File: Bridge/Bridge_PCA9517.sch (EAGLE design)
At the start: 13 parts, among them IC2 SI7005, X1 SCL, X2 3v3, X3 GND, X4 SCL, X5 SDA, X6 SDA, X7 3v3, X8 GND

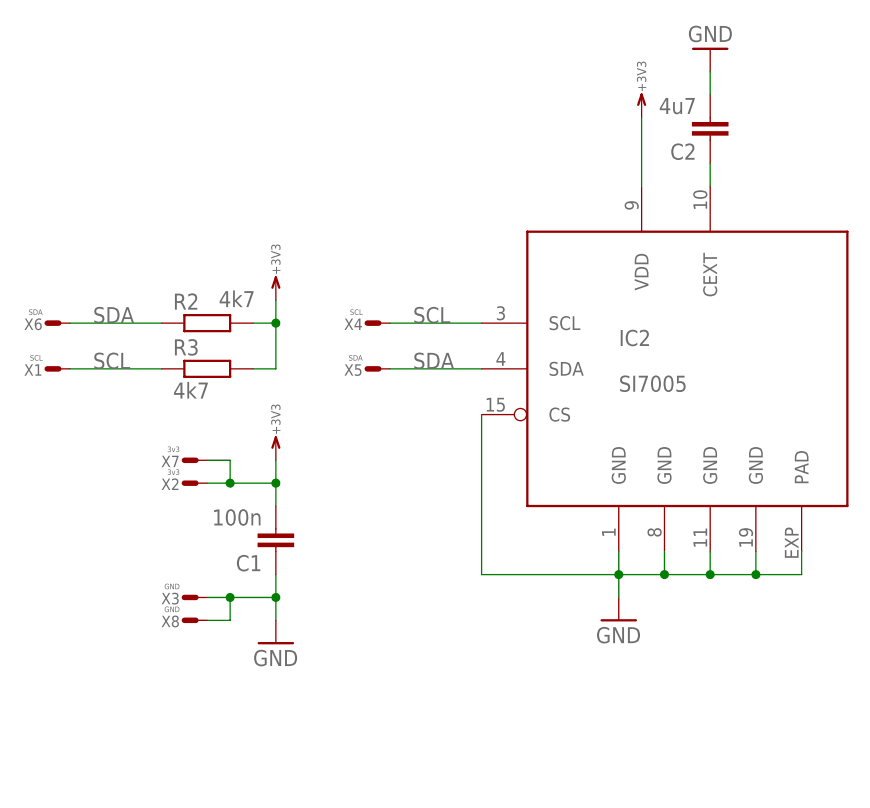
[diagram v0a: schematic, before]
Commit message: Typo correction and more elegance presentation
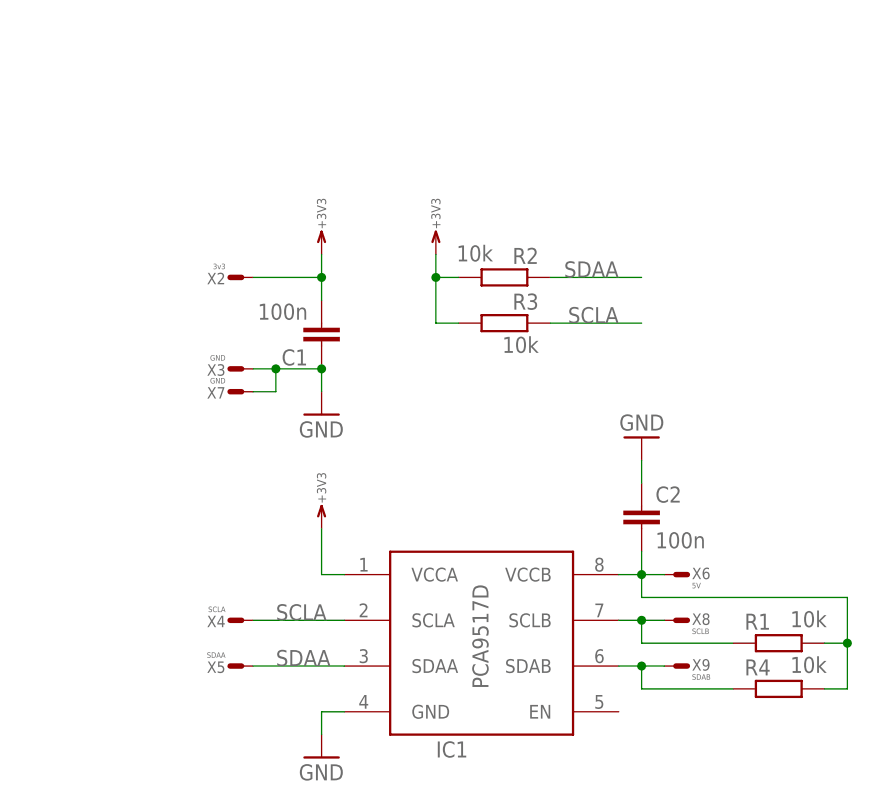
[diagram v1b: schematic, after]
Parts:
- removed IC2: SI7005, Sensors:SI7005
- removed X1: SCL, Conn:WIREPADT1.6/0.9
- added IC1: PCA9517D, Other:PCA9517D
- added R1, R4: 10k, RCL:R0603
- added X9: SDAB, Conn:WIREPADT1.6/0.9
- C2: value 4u7 -> 100n
- R2, R3: value 4k7 -> 10k
- X4: value SCL -> SCLA
- X5: value SDA -> SDAA
- X6: value SDA -> 5V
- X7: value 3v3 -> GND
- X8: value GND -> SCLB
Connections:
- removed net N$1: C2.1, IC2.CEXT
- removed net SCL: IC2.SCL, R3.1, X1.S, X4.S
- removed net SDA: IC2.SDA, R2.1, X5.S, X6.S
- new net N$3: C2.2, IC1.VCCB, R1.2, R4.2, X6.S
- new net SCLA: IC1.SCLA, R3.1, X4.S
- new net SCLB: IC1.SCLB, R1.1, X8.S
- new net SDAA: IC1.SDAA, R2.1, X5.S
- new net SDAB: IC1.SDAB, R4.1, X9.S
- net +3V3: now also IC1.VCCA; no longer IC2.VDD, X7.S
- net GND: now also C2.1, IC1.GND, X7.S; no longer C2.2, IC2.CS, IC2.GND@1, IC2.GND@11, IC2.GND@19, IC2.GND@8, IC2.PAD, X8.S
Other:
- moved on the sheet: C1, C2, R2, R3, X2, X3, X4, X5, X6, X7, X8
